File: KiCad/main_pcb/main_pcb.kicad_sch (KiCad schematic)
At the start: 29 parts, among them U4 SD Card Socket, U5 TI TXB0104DR, U6 TI TXB0104DR, U7 TI TXB0104DR, U9 ILI9488

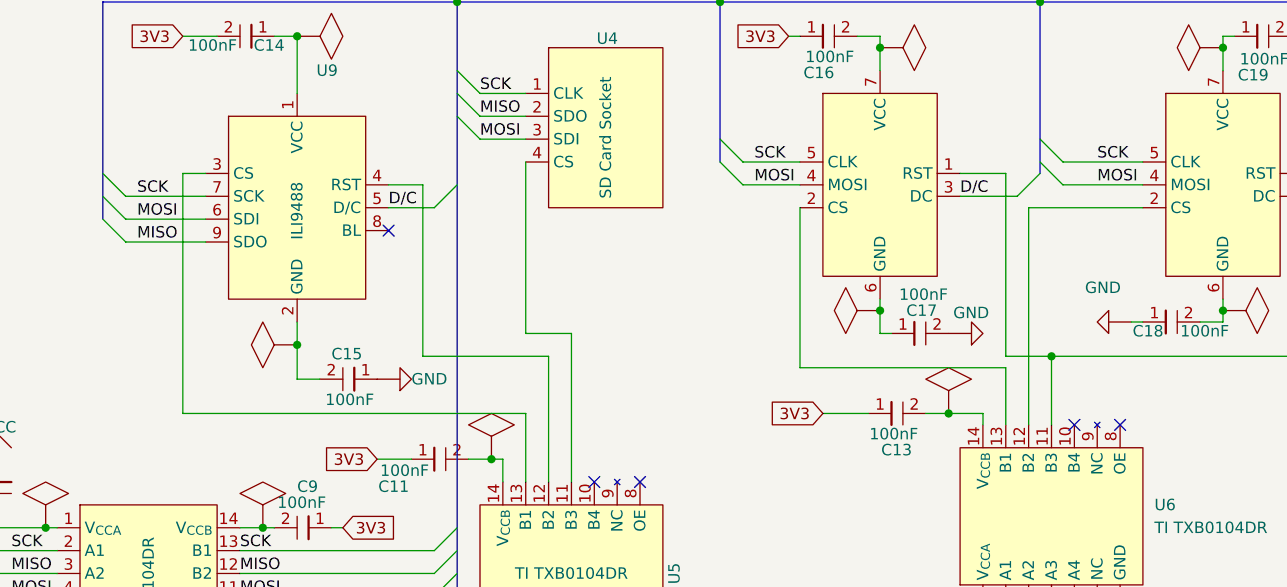
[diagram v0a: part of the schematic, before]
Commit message: feat(KiCad): Continues work on circuit
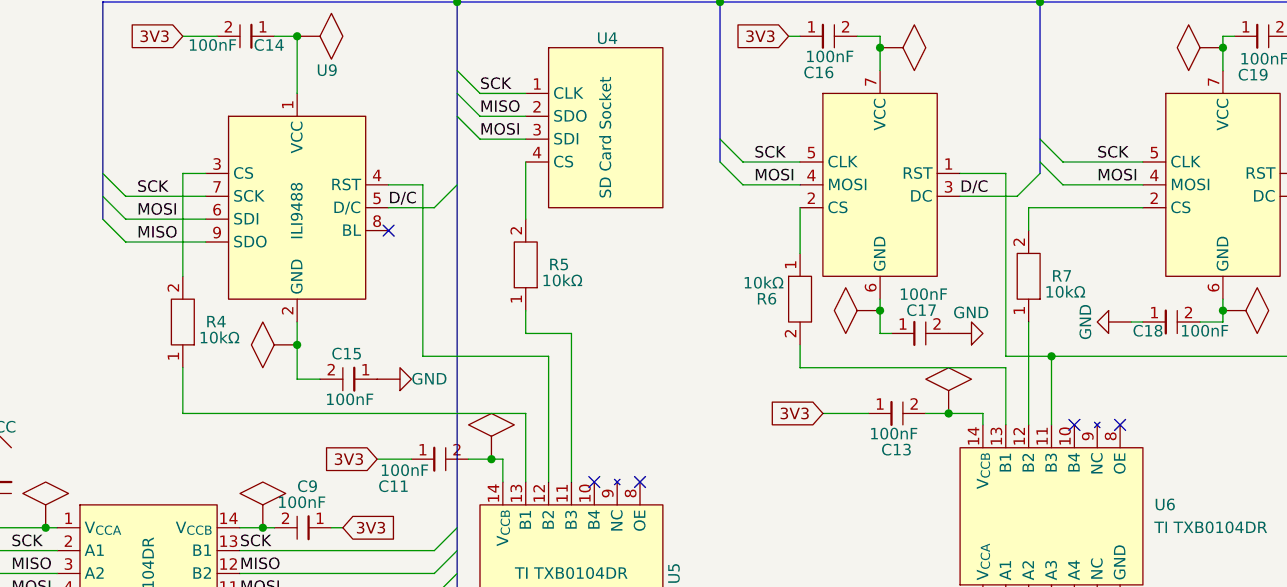
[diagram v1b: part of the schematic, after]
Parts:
- added R4, R5, R6, R7: 10kΩ, symbol lilys_pad:Resistor
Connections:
- net at U2.2 (CS): now also R7.2; no longer U6.12 (B2)
- net at U3.2 (CS): now also R6.1; no longer U6.13 (B1)
- net at U5.11 (B3): now also R5.1; no longer U4.4 (CS)
- net at U5.13 (B1): now also R4.1; no longer U9.3 (CS)
- new net: R5.2, U4.4 (CS)
- new net: R4.2, U9.3 (CS)
- new net: R6.2, U6.13 (B1)
- new net: R7.1, U6.12 (B2)
